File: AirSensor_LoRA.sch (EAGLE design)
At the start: 8 parts, among them U2 RFM95W-915S2

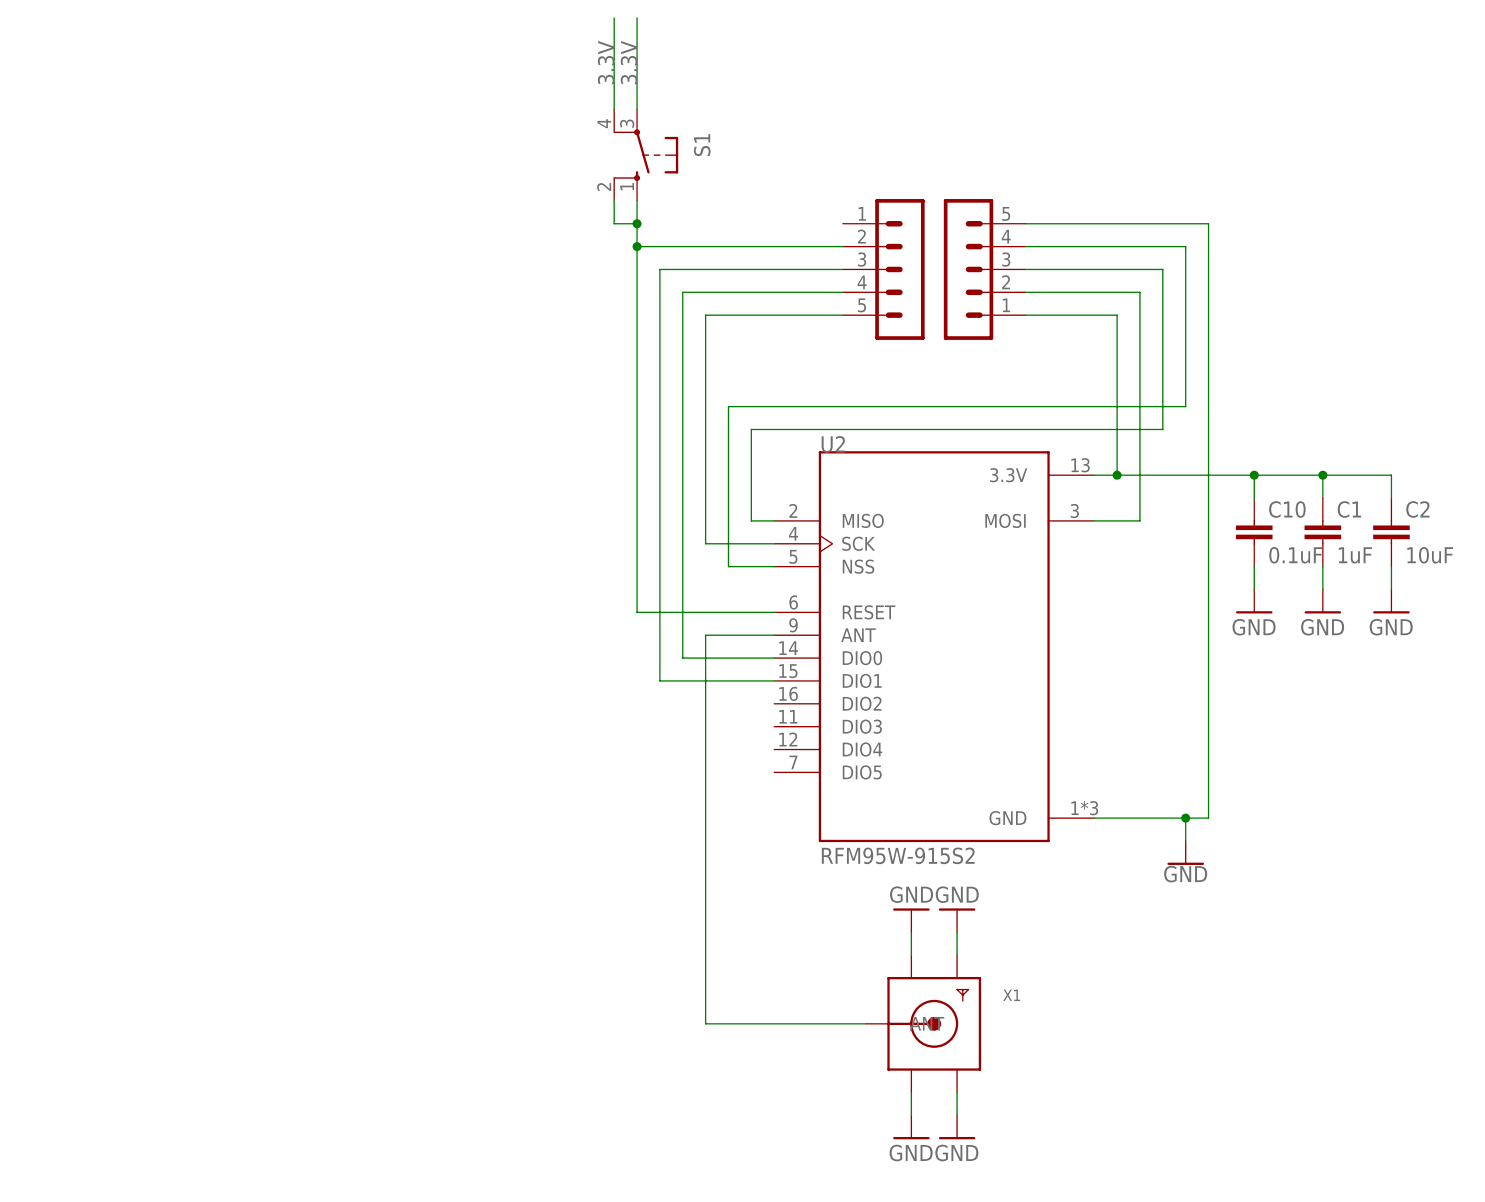
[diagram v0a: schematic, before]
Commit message: nieuw schema lora bordje
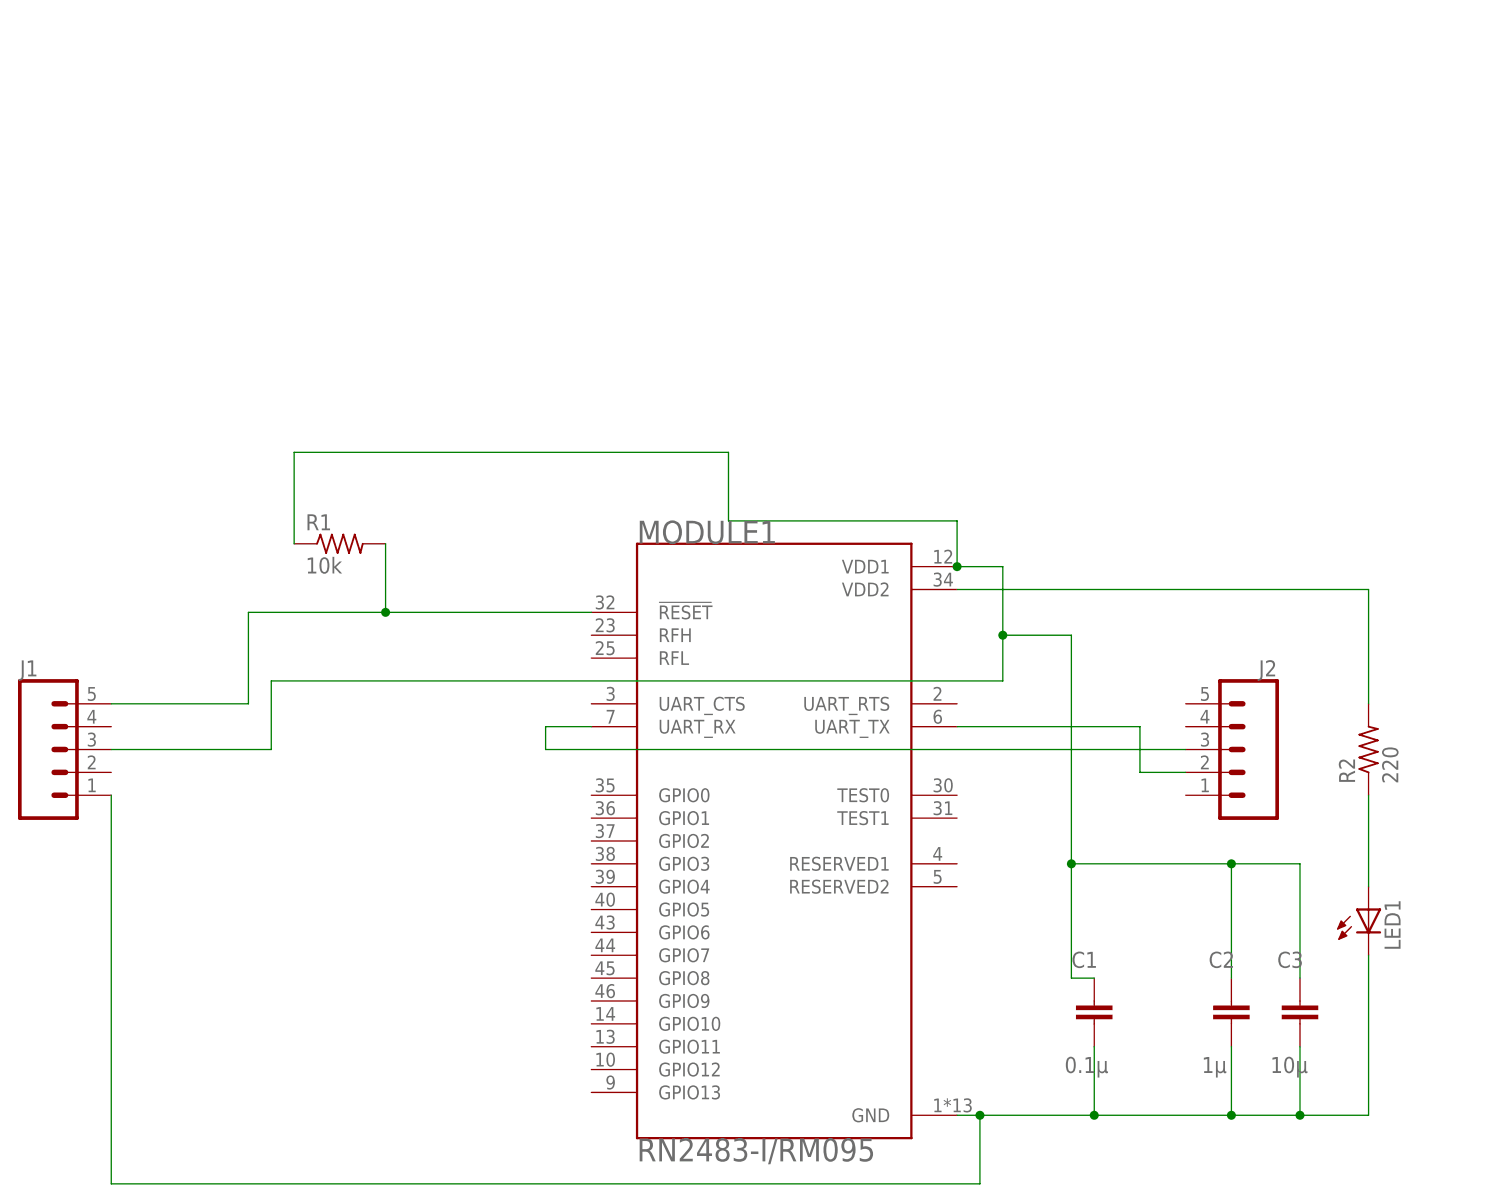
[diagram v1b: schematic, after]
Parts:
- removed C10: 0.1uF, SparkFun-Capacitors:1.0UF-0805-25V-10%
- removed RFM95W_1: LoRa_1, con-lstb:MA05-1
- removed RFM95W_2: LoRa_2, con-lstb:MA05-1
- removed S1: (no value), switch-omron:10-XX
- removed U2: RFM95W-915S2, RFM95W-915S2:RFM95W-915S2
- removed X1: (no value), adafruit:SMACONNECTOR_EDGE
- added C3: 10µ, Resistor_Capacitor:CC0805KRX7R9BB104
- added J1, J2: (no value), SparkFun-Connectors:CONN_05
- added LED1: (no value), adafruit:LEDCHIPLED_0805
- added MODULE1: RN2483-I/RM095, RN2483-I_RM095 (3):RN2483-I/RM095
- added R1: 10k, Resistor_Capacitor:CRCW08050000Z0EA
- added R2: 220, Resistor_Capacitor:CRCW08050000Z0EA
- C1: value 1uF -> 0.1µ; device SparkFun-Capacitors:1.0UF-0805-25V-10% -> Resistor_Capacitor:CC0805KRX7R9BB104
- C2: value 10uF -> 1µ; device SparkFun-Capacitors:1.0UF-0805-25V-10% -> Resistor_Capacitor:CC0805KRX7R9BB104
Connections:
- removed net 3.3V: S1.P, S1.P1
- removed net GND: C1.2, C10.2, C2.2, RFM95W_2.5, U2.GND, X1.GND1, X1.GND2, X1.GND3, X1.GND4
- removed net N$13: RFM95W_1.2, S1.S, S1.S1, U2.RESET
- removed net N$17: C1.1, C10.1, C2.1, RFM95W_2.1, U2.3.3V
- removed net N$18: RFM95W_2.2, U2.MOSI
- removed net N$21: RFM95W_2.3, U2.MISO
- removed net N$22: RFM95W_2.4, U2.NSS
- removed net N$23: RFM95W_1.5, U2.SCK
- removed net N$24: RFM95W_1.4, U2.DIO0
- removed net N$25: RFM95W_1.3, U2.DIO1
- removed net N$26: U2.ANT, X1.ANT
- new net N$1: J2.3, MODULE1.UART_RX
- new net N$2: J2.2, MODULE1.UART_TX
- new net N$3: J1.5, MODULE1.!RESET, R1.2
- new net N$4: C1.1, C2.1, C3.1, J1.3, MODULE1.VDD1, R1.1
- new net N$5: C1.2, C2.2, C3.2, J1.1, LED1.C, MODULE1.GND
- new net N$6: MODULE1.VDD2, R2.2
- new net N$8: LED1.A, R2.1
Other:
- moved on the sheet: C1, C2
